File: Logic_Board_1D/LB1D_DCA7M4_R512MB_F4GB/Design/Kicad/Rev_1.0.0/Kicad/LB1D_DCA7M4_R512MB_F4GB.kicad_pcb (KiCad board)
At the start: 4 copper layers, 50 x 50 mm, 157 parts, among them U1 STM32MP157CAC3, U2 AS4C256M16D3LC-12BCN, U3 S40FC004C1B2C00000, U4 STPMIC1BPQR, U5 DF40C-70DP-0.4V(51), U6 DF40C-70DP-0.4V(51), U7 DF40C-70DP-0.4V(51), U8 WFM200S022XNA3R, U9 BGX220S22HNA21R, X1 32.768kHz, X2 24MHz

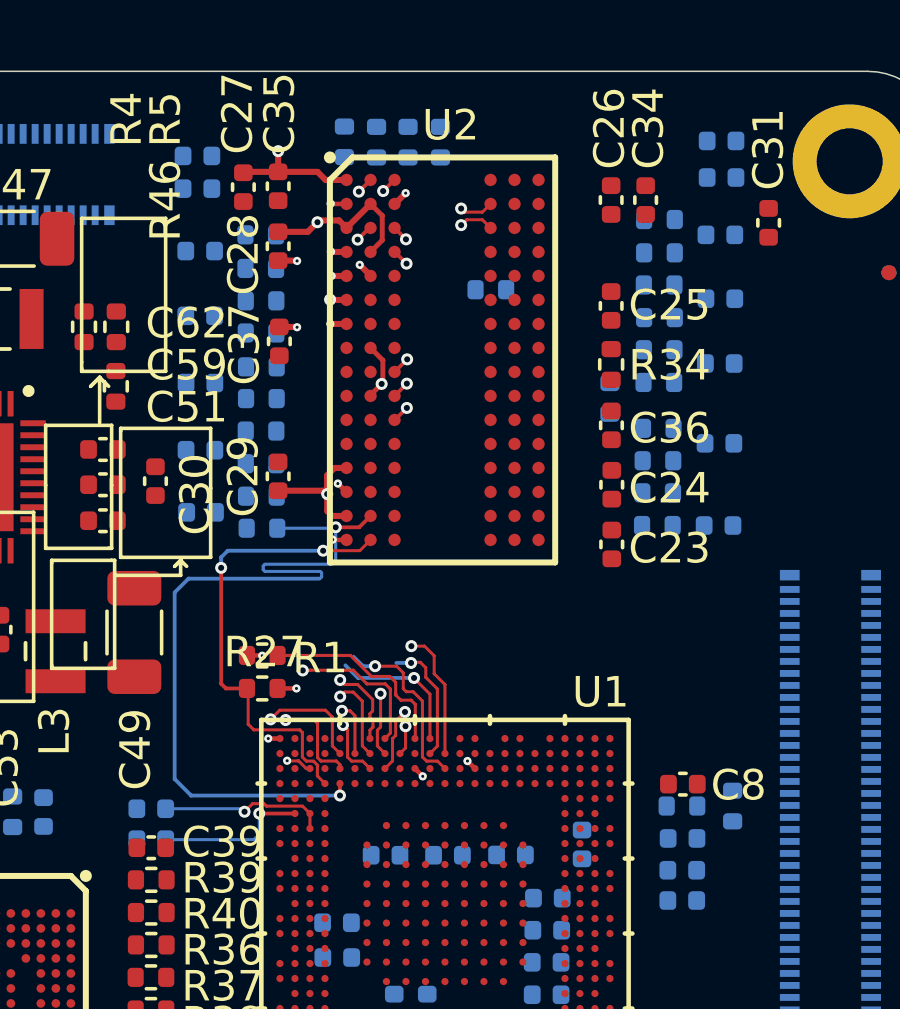
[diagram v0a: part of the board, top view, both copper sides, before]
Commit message: changes
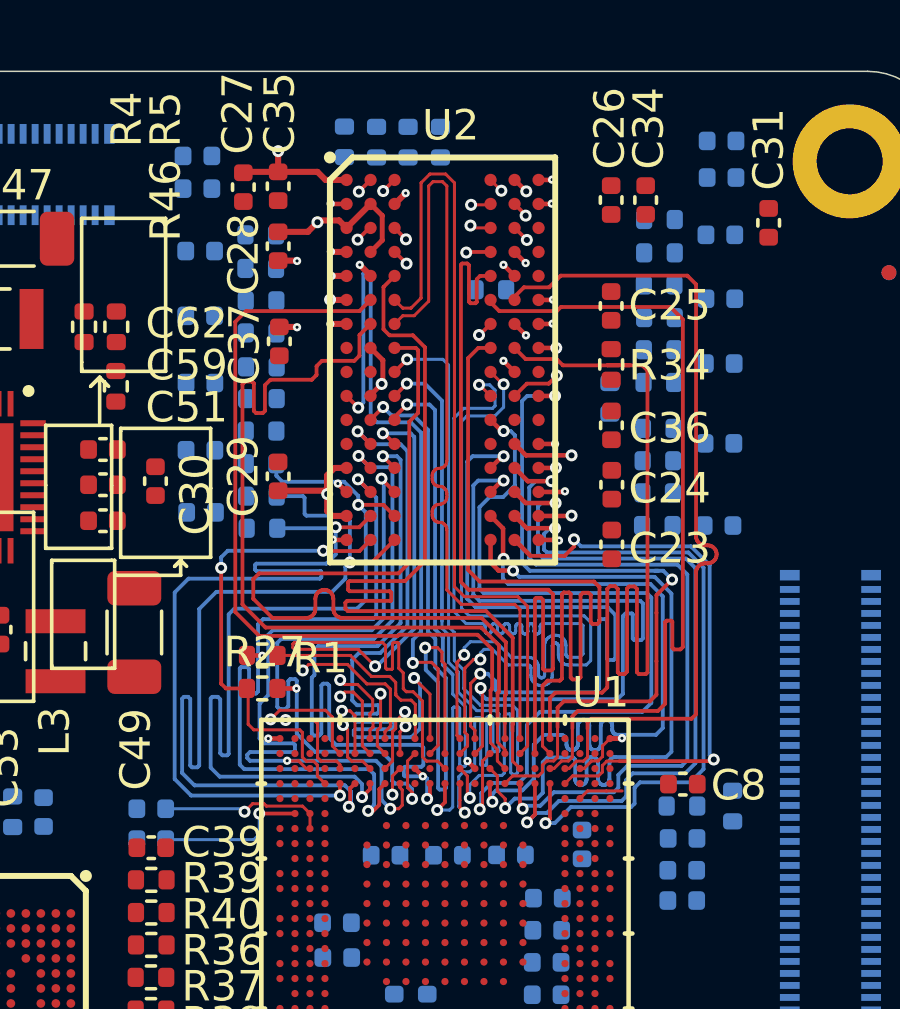
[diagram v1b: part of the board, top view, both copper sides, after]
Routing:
- net DDR_DQ12: track 0.00 -> 32.0 mm
- net DDR_DQ4: track 0.00 -> 31.6 mm, vias 0 -> 2
- net DDR_DQ5: track 0.99 -> 31.6 mm, vias 1 -> 2
- net DDR_A13: track 0.00 -> 30.1 mm, vias 0 -> 2
- net DDR_DQ2: track 2.16 -> 32.1 mm, vias 1 -> 2
- net DDR_A9: track 0.00 -> 28.8 mm, vias 0 -> 2
- net DDR_DQ8: track 0.00 -> 27.8 mm
- net DDR_DQ10: track 0.00 -> 27.8 mm
- net DDR_DQ9: track 0.00 -> 27.7 mm
- net DDR_DQ13: track 0.00 -> 27.7 mm
- net DDR_DQS1_N: track 0.00 -> 27.6 mm
- net DDR_DQ15: track 0.00 -> 27.6 mm
- net DDR_DQ14: track 0.00 -> 27.6 mm
- net DDR_DQ11: track 0.00 -> 27.6 mm
- net DDR_DQM1: track 0.00 -> 27.5 mm
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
